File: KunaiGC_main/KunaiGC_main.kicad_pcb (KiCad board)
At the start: 2 copper layers, 15.5 x 48.5 mm, 19 parts, among them J1 Conn_01x06, J2 Conn_01x01, J3 Conn_02x04_Counter_Clockwise, J4 Conn_02x04_Counter_Clockwise, J5 Conn_01x06, U1 XC9536VQ44, U2 M25P40

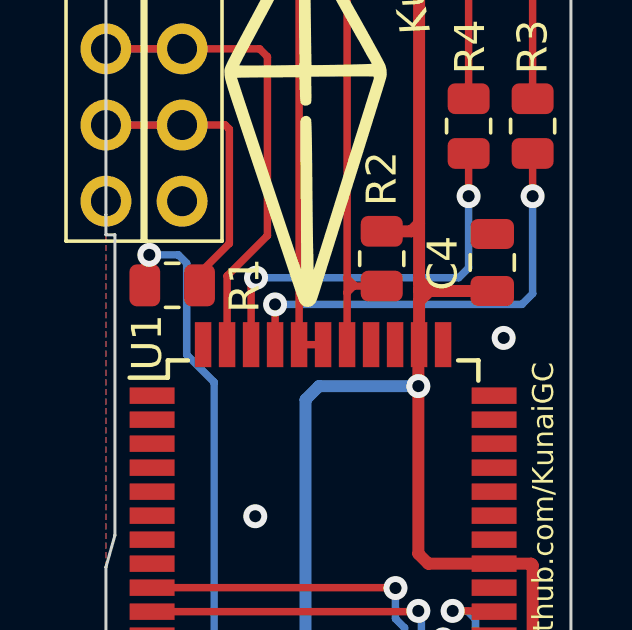
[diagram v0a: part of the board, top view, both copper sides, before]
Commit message: updated to latest files
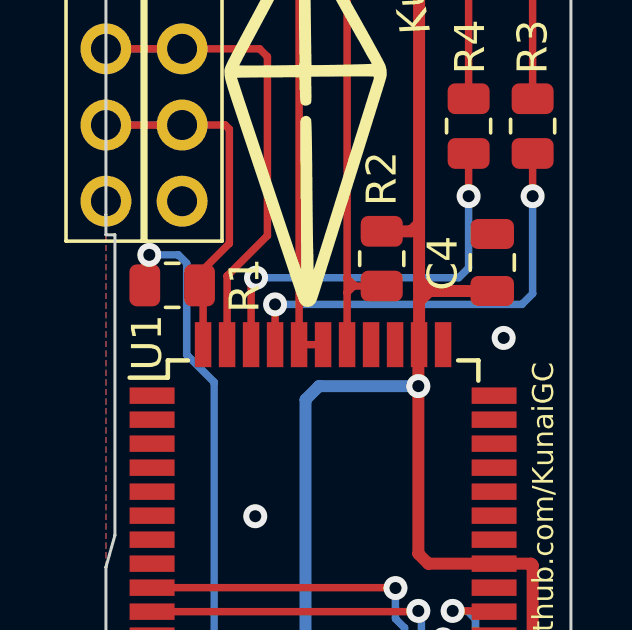
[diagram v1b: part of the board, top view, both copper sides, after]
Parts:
- R3, R4: value 1k -> 470
- RN1: value R_Pack04 -> 10k
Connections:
- U1 pad 44: unconnected-(U1-Pad44) -> EXI.CLK
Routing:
- net EXI.CLK: track 12.1 -> 14.1 mm
